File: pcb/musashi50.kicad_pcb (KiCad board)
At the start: 2 copper layers, 160 x 140 mm, 68 parts, among them J1 MJ-4PP-9, U1 ProMicro_r, U2 joystick

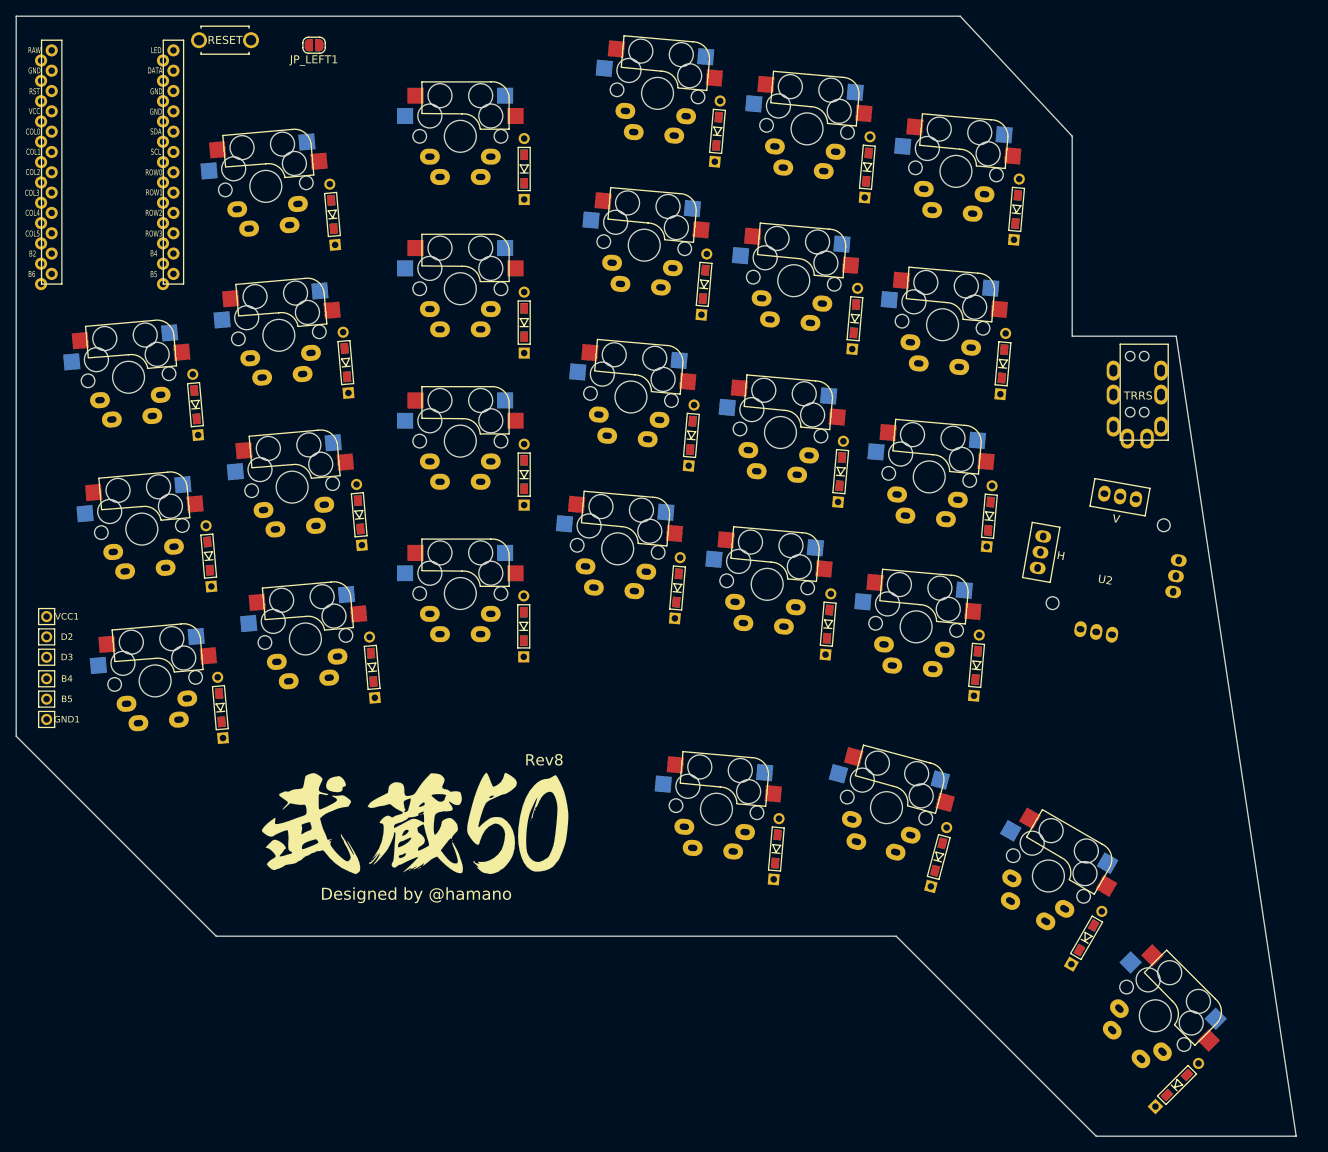
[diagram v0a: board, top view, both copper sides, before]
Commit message: update rev9
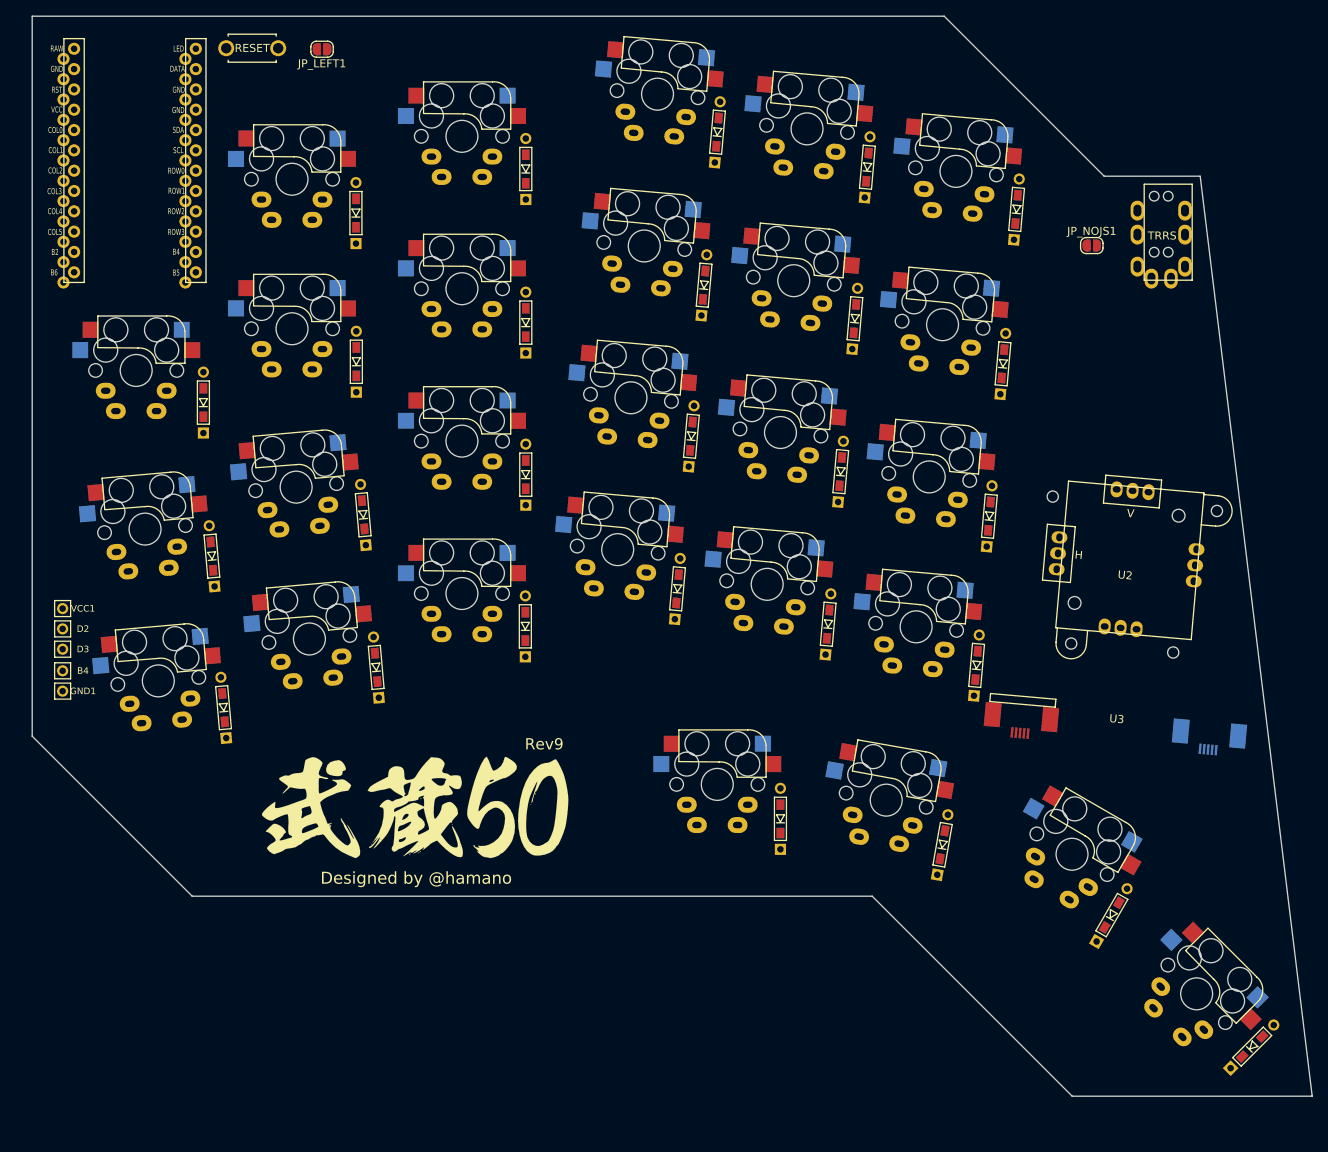
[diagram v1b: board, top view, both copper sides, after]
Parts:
- removed B5: MountingHole_Pad, foostan:1pin_conn
- added JP_NOJS1: Jumper, Jumper:SolderJumper-2_P1.3mm_Open_RoundedPad1.0x1.5mm, F.Cu at (171.5, 41.7)
- added U3: joystick_s, local:Joycon_Stick, F.Cu at (176.2, 81.0)
- moved J1 20.2 mm to (181.0, 34.0)
- moved D_A5 10.6 mm to (191.5, 141.8)
- moved SW_A5 5.85 mm to (184.6, 135.2)
- moved D_B5 4.24 mm to (174.0, 125.4)
- moved GND1 4.07 mm to (42.8, 97.4)
- moved SW_B5 4.01 mm to (169.0, 117.8)
- moved D_D5 3.81 mm to (132.5, 113.3), turned to 90 degrees
- moved SW_RST1 3.54 mm to (66.5, 17.0)
- moved SW_E1 3.39 mm to (71.5, 33.4), turned to 0 degrees
- moved SW_D5 3.10 mm to (124.6, 109.0), turned to 0 degrees
- moved D_E1 2.94 mm to (79.5, 37.6), turned to 90 degrees
- moved U1 2.81 mm to (51.8, 31.6)
- moved U2 2.38 mm to (175.8, 80.9), turned to 355 degrees
- moved B4 2.24 mm to (42.8, 94.8)
- moved D2 2.24 mm to (42.8, 89.6)
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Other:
- board size 160 x 140 mm -> 160 x 135 mm
- net class Default: clearance 0.23 -> 0.2
- rule pad_to_mask_clearance: 0.05 -> 0
- rule trace_clearance: 0.23 -> 0.2
- board text added: "Rev9"
- board text removed: "Rev8"
